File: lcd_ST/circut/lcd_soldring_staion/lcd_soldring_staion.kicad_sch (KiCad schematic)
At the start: 42 parts, among them J1 DIN-5, J2 Conn_01x05_Pin, J3 Conn_01x01_Pin, J4 Conn_01x01_Pin, J44 Screw_Terminal_01x02, J5 Conn_01x01_Pin, J6 Conn_01x01_Pin, J7 Conn_01x04_Pin, J8 Conn_01x04_Pin, J9 Conn_01x04_Pin, Q2 Si4162DY, SW1 SW_Push, U1 PIC16F15223T-I/SL, U2 L7805, U3 LM358

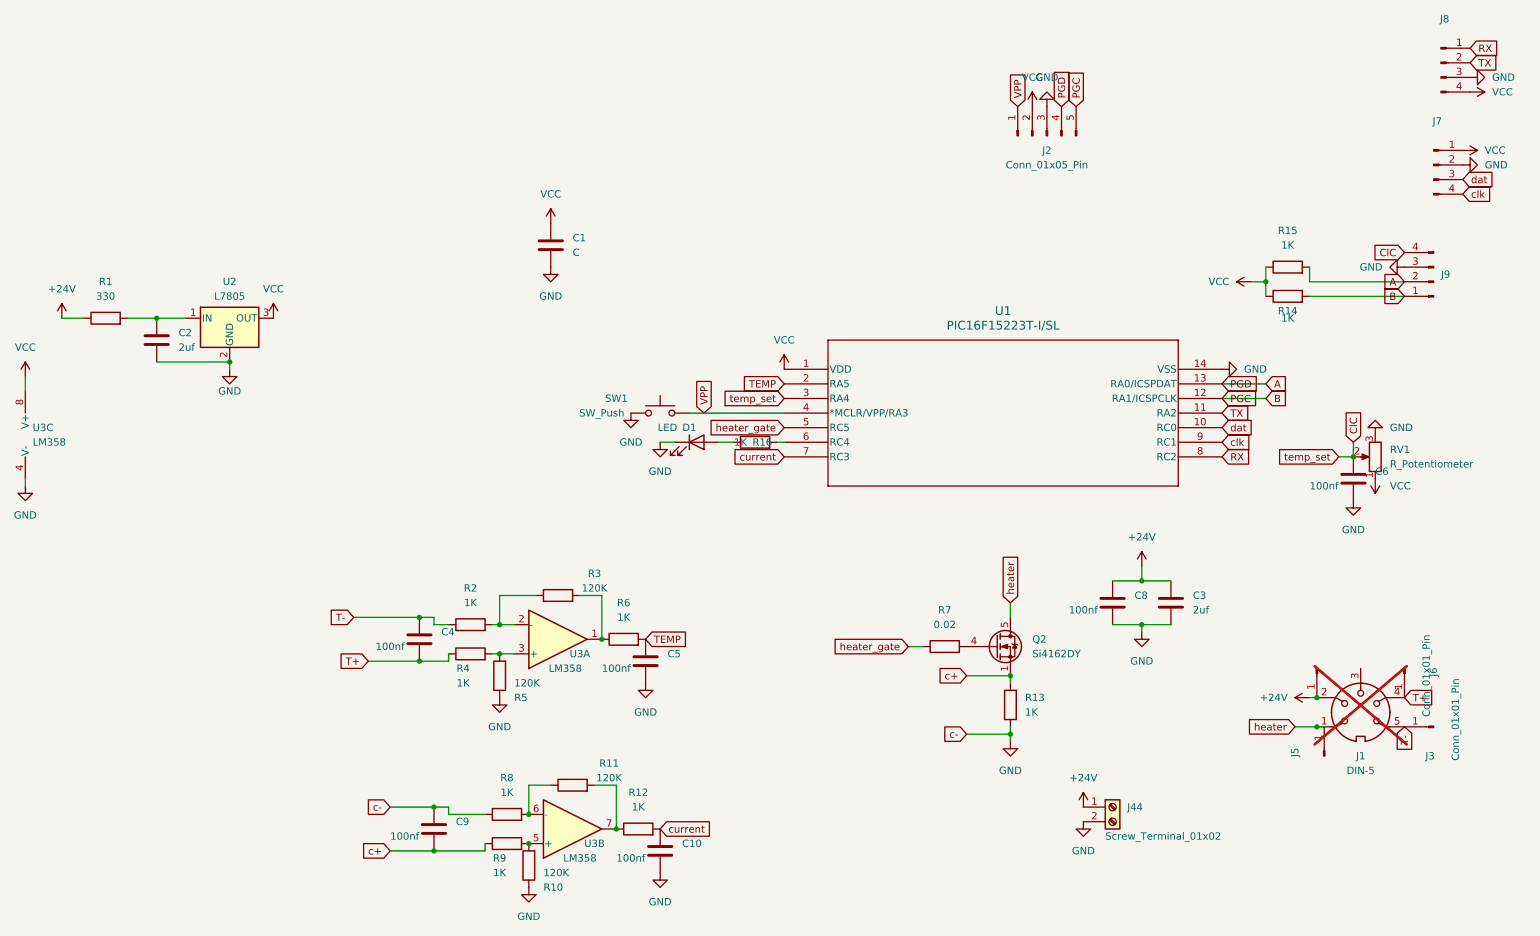
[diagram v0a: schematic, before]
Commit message: pcb v2
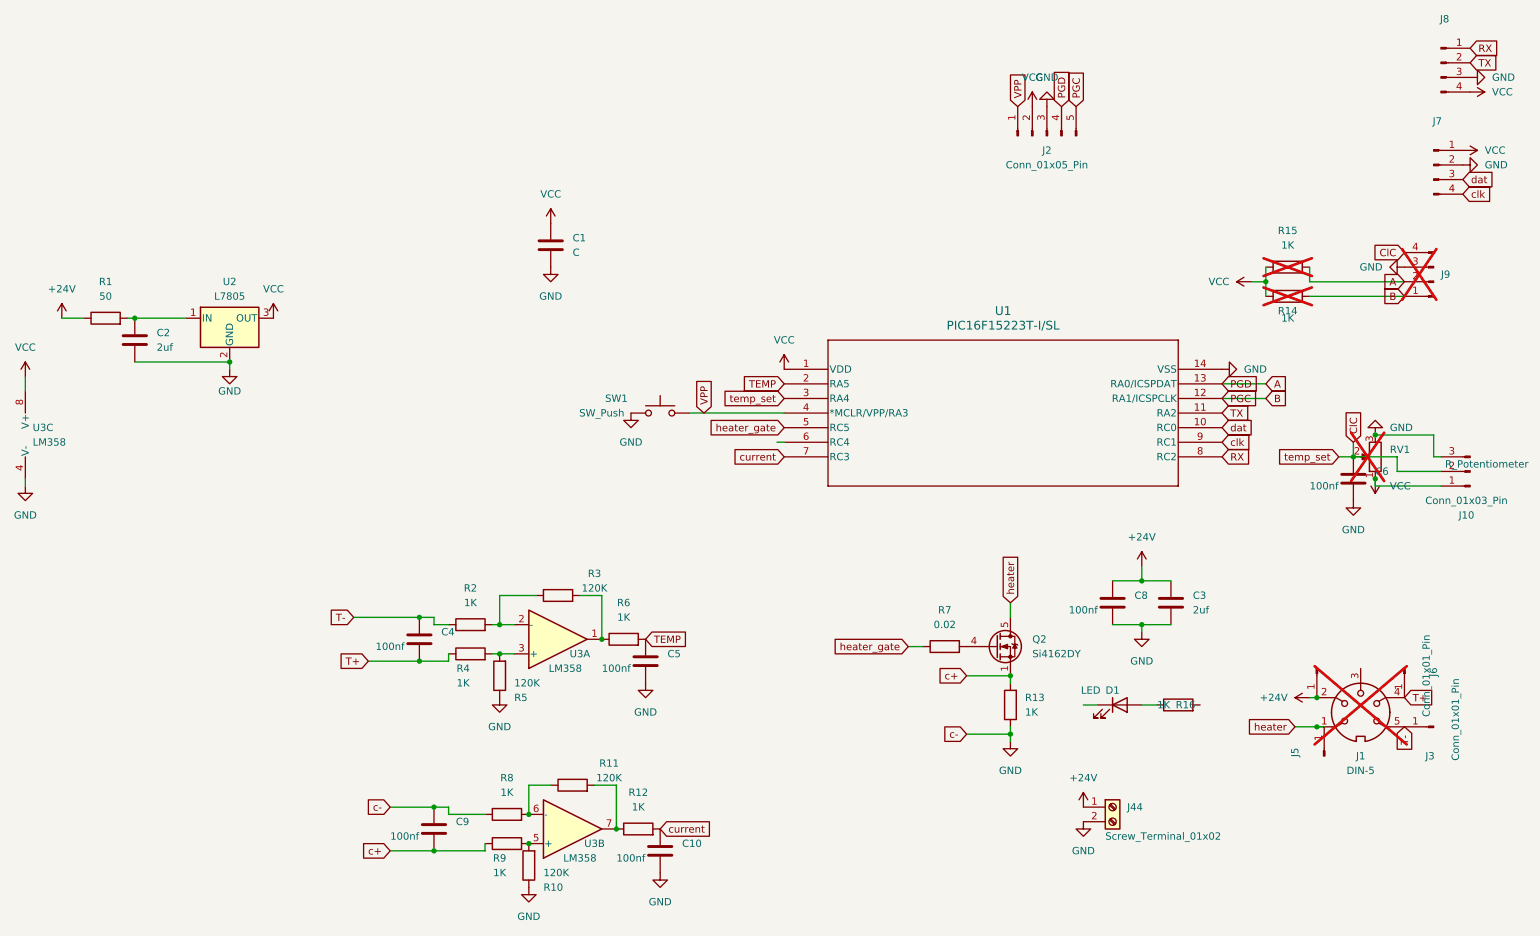
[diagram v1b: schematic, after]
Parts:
- added J10: Conn_01x03_Pin, symbol Connector:Conn_01x03_Pin
- J9, R15: now not fitted; now left out of the parts list
- R1: value 330 -> 50; footprint Resistor_SMD:R_0805_2012Metric_Pad1.20x1.40mm_HandSolder -> Resistor_THT:R_Axial_DIN0207_L6.3mm_D2.5mm_P7.62mm_Horizontal
- R14, RV1: now not fitted
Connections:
- net ClC: now also J10.2 (Pin_2)
- net GND: now also J10.3 (Pin_3); no longer D1.1 (K)
- net VCC: now also J10.1 (Pin_1)
- net at R16.2: no longer U1.6 (RC4)
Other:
- moved on the sheet: C2, D1, R16

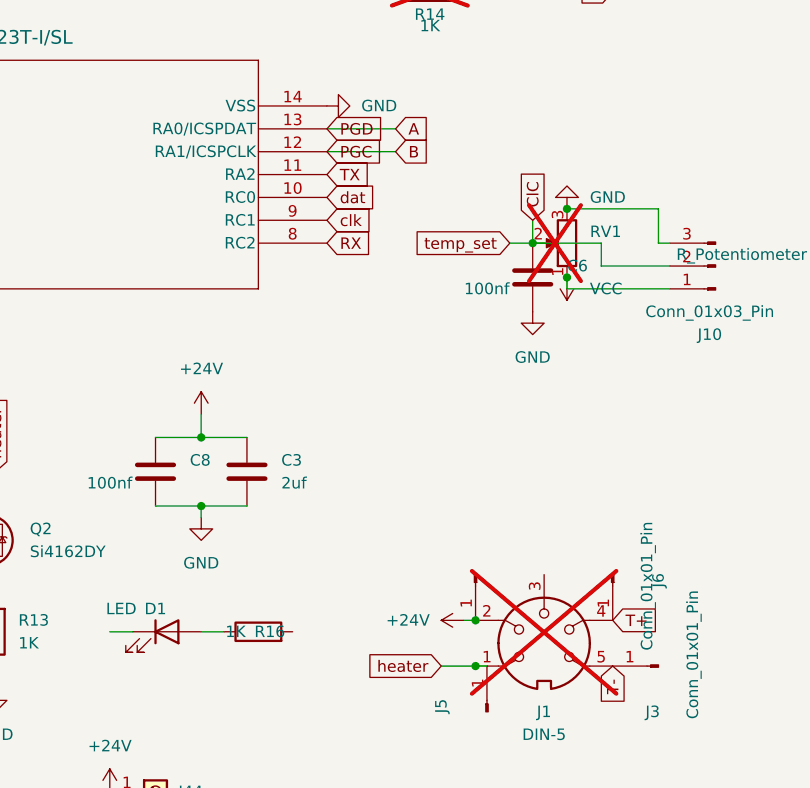
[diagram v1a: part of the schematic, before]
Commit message: pcbing
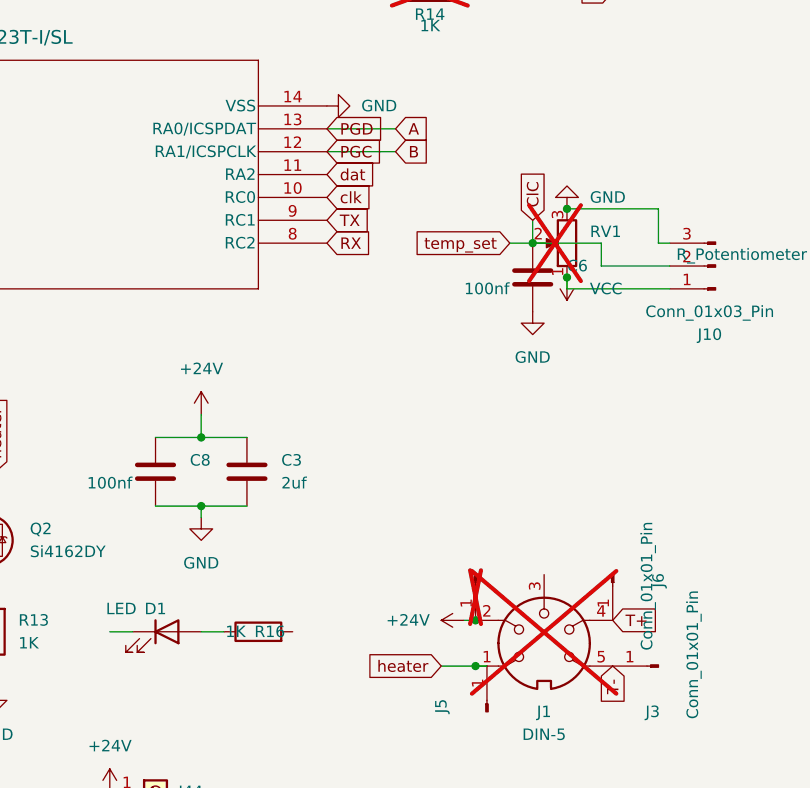
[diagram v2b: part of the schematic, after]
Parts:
- J4: now not fitted; now left out of the parts list
- J7, J8: footprint Connector:FanPinHeader_1x04_P2.54mm_Vertical -> Connector:01x04_fat_pins
- R14: now left out of the parts list
- U3: footprint Package_SO:SOIC-8_5.3x6.2mm_P1.27mm -> Package_SO:SOIC-8_3.9x4.9mm_P1.27mm
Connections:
- net TX: now also U1.9 (RC1); no longer U1.11 (RA2)
- net clk: now also U1.10 (RC0); no longer U1.9 (RC1)
- net dat: now also U1.11 (RA2); no longer U1.10 (RC0)
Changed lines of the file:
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@@
 		)
 	)
-	(global_label "TX"
-		(shape input)
-		(at 232.41 81.28 0)
-		(fields_autoplaced yes)
-		(effects
-			(font
-				(size 1.27 1.27)
-			)
-			(justify left)
-		)
-		(property "Intersheetrefs" "${INTERSHEET_REFS}"
-			(at 237.5723 81.28 0)
-			(effects
-				(font
-					(size 1.27 1.27)
-				)
-				(justify left)
-				(hide yes)
-			)
-		)
-	)
 	(global_label "heater"
 		(shape input)
@@
 		)
 	)
-	(global_label "clk"
+	(global_label "A"
 		(shape input)
-		(at 232.41 86.36 0)
+		(at 240.03 76.2 0)
 		(fields_autoplaced yes)
 		(effects
@@
 		)
 		(property "Intersheetrefs" "${INTERSHEET_REFS}"
-			(at 238.1771 86.36 0)
+			(at 244.1038 76.2 0)
 			(effects
 				(font
@@
 		)
 	)
-	(global_label "A"
+	(global_label "temp_set"
 		(shape input)
-		(at 240.03 76.2 0)
+		(at 156.21 78.74 180)
+		(fields_autoplaced yes)
+		(effects
+			(font
+				(size 1.27 1.27)
+			)
+			(justify right)
+		)
+		(property "Intersheetrefs" "${INTERSHEET_REFS}"
+			(at 144.7582 78.74 0)
+			(effects
+				(font
+					(size 1.27 1.27)
+				)
+				(justify right)
+				(hide yes)
+			)
+		)
+	)
+	(global_label "TEMP"
+		(shape input)
+		(at 132.08 120.65 0)
 		(fields_autoplaced yes)
 		(effects
@@
 		)
 		(property "Intersheetrefs" "${INTERSHEET_REFS}"
-			(at 244.1038 76.2 0)
+			(at 139.9032 120.65 0)
 			(effects
 				(font
@@
 		)
 	)
-	(global_label "temp_set"
+	(global_label "c+"
 		(shape input)
-		(at 156.21 78.74 180)
+		(at 187.96 127 180)
 		(fields_autoplaced yes)
 		(effects
@@
 		)
 		(property "Intersheetrefs" "${INTERSHEET_REFS}"
-			(at 144.7582 78.74 0)
+			(at 182.3138 127 0)
 			(effects
 				(font
@@
 		)
 	)
-	(global_label "TEMP"
+	(global_label "TX"
 		(shape input)
-		(at 132.08 120.65 0)
+		(at 232.41 86.36 0)
 		(fields_autoplaced yes)
 		(effects
@@
 		)
 		(property "Intersheetrefs" "${INTERSHEET_REFS}"
-			(at 139.9032 120.65 0)
+			(at 237.5723 86.36 0)
 			(effects
 				(font
@@
 		)
 	)
-	(global_label "c+"
+	(global_label "TEMP"
 		(shape input)
-		(at 187.96 127 180)
+		(at 156.21 76.2 180)
 		(fields_autoplaced yes)
 		(effects
@@
 		)
 		(property "Intersheetrefs" "${INTERSHEET_REFS}"
-			(at 182.3138 127 0)
+			(at 148.3868 76.2 0)
 			(effects
 				(font
@@
 		)
 	)
-	(global_label "TEMP"
+	(global_label "dat"
 		(shape input)
-		(at 156.21 76.2 180)
+		(at 232.41 81.28 0)
 		(fields_autoplaced yes)
 		(effects
@@
 				(size 1.27 1.27)
 			)
-			(justify right)
+			(justify left)
 		)
 		(property "Intersheetrefs" "${INTERSHEET_REFS}"
-			(at 148.3868 76.2 0)
+			(at 238.4189 81.28 0)
 			(effects
 				(font
 					(size 1.27 1.27)
 				)
-				(justify right)
+				(justify left)
+				(hide yes)
+			)
+		)
+	)
+	(global_label "clk"
+		(shape input)
+		(at 232.41 83.82 0)
+		(fields_autoplaced yes)
+		(effects
+			(font
+				(size 1.27 1.27)
+			)
+			(justify left)
+		)
+		(property "Intersheetrefs" "${INTERSHEET_REFS}"
+			(at 238.1771 83.82 0)
+			(effects
+				(font
+					(size 1.27 1.27)
+				)
+				(justify left)
 				(hide yes)
 			)
@@
 		)
 	)
-	(global_label "dat"
-		(shape input)
-		(at 232.41 83.82 0)
-		(fields_autoplaced yes)
-		(effects
-			(font
-				(size 1.27 1.27)
-			)
-			(justify left)
-		)
-		(property "Intersheetrefs" "${INTERSHEET_REFS}"
-			(at 238.4189 83.82 0)
-			(effects
-				(font
-					(size 1.27 1.27)
-				)
-				(justify left)
-				(hide yes)
-			)
-		)
-	)
 	(global_label "PGD"
 		(shape input)
@@
 			)
 		)
-		(property "Footprint" "Package_SO:SOIC-8_5.3x6.2mm_P1.27mm"
+		(property "Footprint" "Package_SO:SOIC-8_3.9x4.9mm_P1.27mm"
 			(at 119.38 153.67 0)
 			(effects
@@
 			)
 		)
-		(property "Footprint" "Connector:FanPinHeader_1x04_P2.54mm_Vertical"
+		(property "Footprint" "Connector:01x04_fat_pins"
 			(at 270.51 20.32 0)
 			(effects
@@
 		(at 243.84 60.96 90)
 		(unit 1)
-		(exclude_from_sim no)
-		(in_bom yes)
-		(on_board yes)
+		(exclude_from_sim yes)
+		(in_bom no)
+		(on_board no)
 		(dnp yes)
 		(property "Reference" "R14"
@@
 			)
 		)
-		(property "Footprint" "Connector:FanPinHeader_1x04_P2.54mm_Vertical"
+		(property "Footprint" "Connector:01x04_fat_pins"
 			(at 269.24 38.1 0)
 			(effects
@@
 			)
 		)
-		(property "Footprint" "Package_SO:SOIC-8_5.3x6.2mm_P1.27mm"
+		(property "Footprint" "Package_SO:SOIC-8_3.9x4.9mm_P1.27mm"
 			(at 26.67 85.09 0)
 			(effects
@@
 			)
 		)
-		(property "Footprint" "Package_SO:SOIC-8_5.3x6.2mm_P1.27mm"
+		(property "Footprint" "Package_SO:SOIC-8_3.9x4.9mm_P1.27mm"
 			(at 116.84 120.65 0)
 			(effects
@@
 		(unit 1)
 		(exclude_from_sim no)
-		(in_bom yes)
-		(on_board yes)
-		(dnp no)
+		(in_bom no)
+		(on_board no)
+		(dnp yes)
 		(property "Reference" "J4"
 			(at 254 126.365 0)

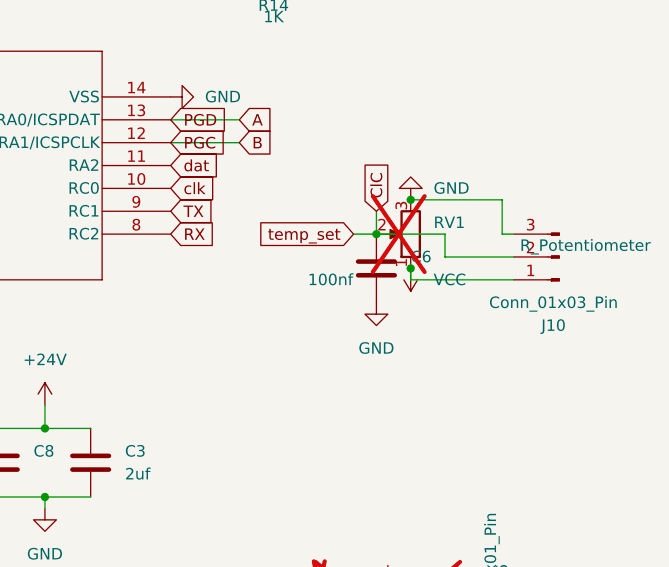
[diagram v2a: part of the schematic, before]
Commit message: da
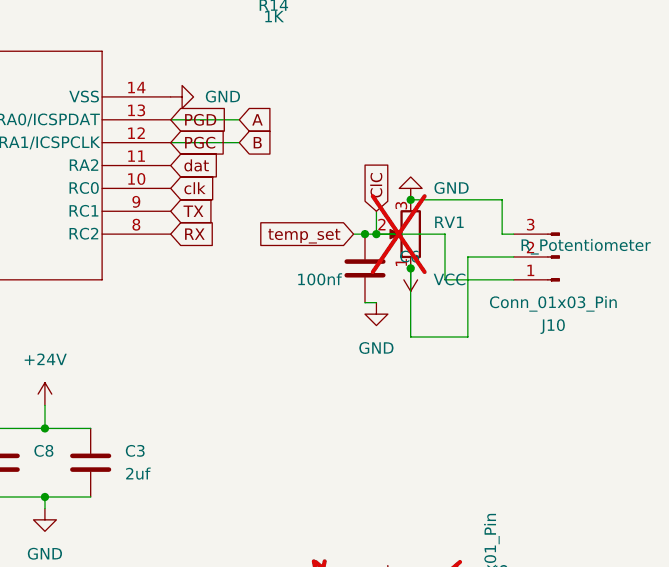
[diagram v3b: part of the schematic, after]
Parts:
- J10: footprint (none) -> Connector:FanPinHeader_1x03_P2.54mm_Vertical
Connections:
- net ClC: now also J10.1 (Pin_1); no longer J10.2 (Pin_2)
- net VCC: now also J10.2 (Pin_2); no longer J10.1 (Pin_1)
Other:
- moved on the sheet: C6
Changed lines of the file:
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@@
 	)
 	(junction
+		(at 254 88.9)
+		(diameter 0)
+		(color 0 0 0 0)
+	)
+	(junction
 		(at 92.71 124.46)
 		(diameter 0)
@@
 	(wire
 		(pts
+			(xy 254 96.52) (xy 255.27 96.52)
+		)
+		(stroke
+			(width 0)
+			(type default)
+		)
+	)
+	(wire
+		(pts
 			(xy 41.91 64.77) (xy 43.18 64.77)
 		)
@@
 	(wire
 		(pts
+			(xy 265.43 100.33) (xy 259.08 100.33)
+		)
+		(stroke
+			(width 0)
+			(type default)
+		)
+	)
+	(wire
+		(pts
 			(xy 270.51 88.9) (xy 269.24 88.9)
 		)
@@
 	(wire
 		(pts
-			(xy 270.51 91.44) (xy 262.89 91.44)
+			(xy 270.51 93.98) (xy 262.89 93.98)
 		)
 		(stroke
@@
 	(wire
 		(pts
+			(xy 270.51 91.44) (xy 265.43 91.44)
+		)
+		(stroke
+			(width 0)
+			(type default)
+		)
+	)
+	(wire
+		(pts
 			(xy 139.7 81.28) (xy 156.21 81.28)
 		)
@@
 	(wire
 		(pts
-			(xy 259.08 92.71) (xy 259.08 93.98)
+			(xy 259.08 92.71) (xy 259.08 100.33)
+		)
+		(stroke
+			(width 0)
+			(type default)
+		)
+	)
+	(wire
+		(pts
+			(xy 262.89 88.9) (xy 262.89 93.98)
 		)
 		(stroke
@@
 	(wire
 		(pts
-			(xy 247.65 60.96) (xy 264.16 60.96)
+			(xy 265.43 91.44) (xy 265.43 100.33)
 		)
 		(stroke
@@
 	(wire
 		(pts
-			(xy 270.51 93.98) (xy 259.08 93.98)
+			(xy 247.65 60.96) (xy 264.16 60.96)
 		)
 		(stroke
@@
 	(wire
 		(pts
+			(xy 254 88.9) (xy 255.27 88.9)
+		)
+		(stroke
+			(width 0)
+			(type default)
+		)
+	)
+	(wire
+		(pts
 			(xy 240.03 55.88) (xy 240.03 58.42)
 		)
@@
 	(wire
 		(pts
-			(xy 252.73 88.9) (xy 255.27 88.9)
+			(xy 252.73 88.9) (xy 254 88.9)
 		)
 		(stroke
@@
 	(wire
 		(pts
-			(xy 262.89 91.44) (xy 262.89 88.9)
-		)
-		(stroke
-			(width 0)
-			(type default)
-		)
-	)
-	(wire
-		(pts
 			(xy 92.71 124.46) (xy 97.79 124.46)
 		)
@@
 			)
 		)
-		(property "Footprint" ""
+		(property "Footprint" "Connector:FanPinHeader_1x03_P2.54mm_Vertical"
 			(at 275.59 91.44 0)
 			(effects
@@
 	(symbol
 		(lib_id "Device:C")
-		(at 255.27 92.71 0)
+		(at 254 92.71 0)
 		(unit 1)
 		(exclude_from_sim no)
@@
 		(dnp no)
 		(property "Reference" "C6"
-			(at 259.08 91.4399 0)
+			(at 257.81 91.4399 0)
 			(effects
 				(font
@@
 		)
 		(property "Value" "100nf"
-			(at 247.65 93.98 0)
+			(at 246.38 93.98 0)
 			(effects
 				(font
@@
 		)
 		(property "Footprint" "Capacitor_SMD:C_1206_3216Metric_Pad1.33x1.80mm_HandSolder"
-			(at 256.2352 96.52 0)
+			(at 254.9652 96.52 0)
 			(effects
 				(font
@@
 		)
 		(property "Datasheet" "~"
-			(at 255.27 92.71 0)
+			(at 254 92.71 0)
 			(effects
 				(font
@@
 		)
 		(property "Description" "Unpolarized capacitor"
-			(at 255.27 92.71 0)
+			(at 254 92.71 0)
 			(effects
 				(font
